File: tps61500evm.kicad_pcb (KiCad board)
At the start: 2 copper layers, 46 x 25 mm, 18 parts, among them J1 Vin, J2 PWM, J3 OVP_Resistor(R1), J4 EN_DIMC, J5 LEDs, J6 FB Resistor, U1 TPS61500PWPR

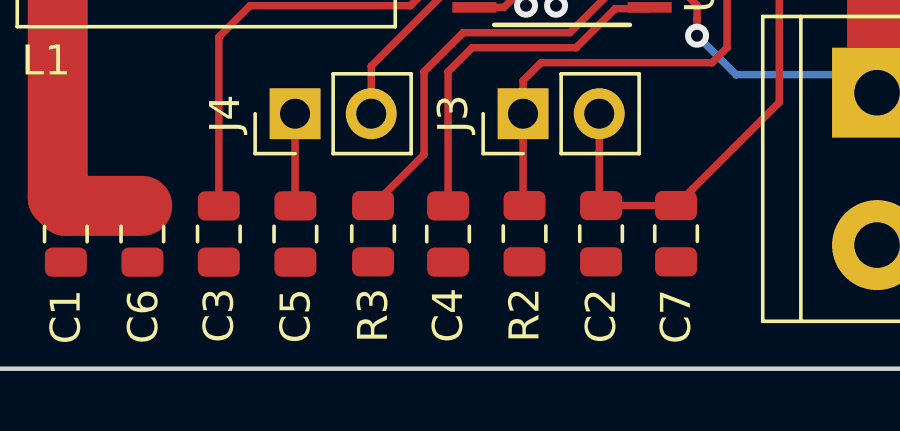
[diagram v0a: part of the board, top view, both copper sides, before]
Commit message: Updated files
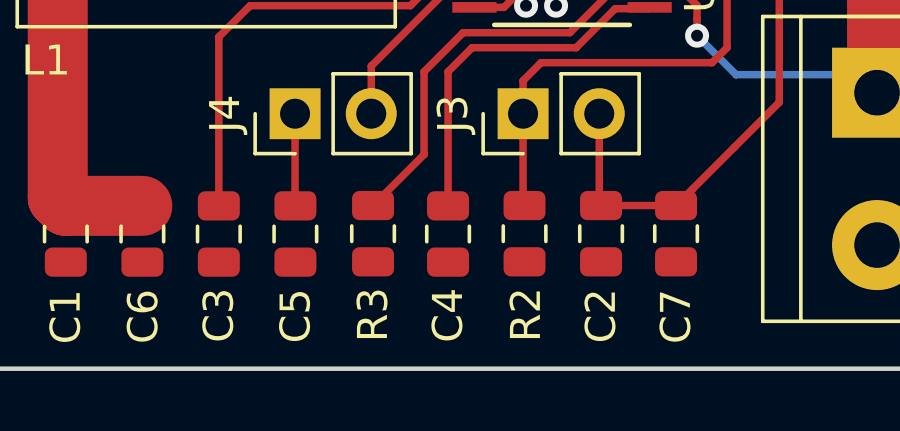
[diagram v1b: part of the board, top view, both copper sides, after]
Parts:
- R2, R3: footprint Capacitor_SMD:C_0805_2012Metric -> Resistor_SMD:R_0805_2012Metric
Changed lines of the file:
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@@
     (add_net "Net-(R3-Pad1)")
+  )
+  (module Resistor_SMD:R_0805_2012Metric (layer F.Cu)
+    (at 45.3 35.5 270)
+    (descr "Resistor SMD 0805 (2012 Metric), square (rectangular) end terminal, IPC_7351 nominal, (Body size source: https://docs.google.com/spreadsheets/d/1BsfQQcO9C6DZCsRaXUlFlo91Tg2WpOkGARC1WS5S8t0/edit?usp=sharing), generated with kicad-footprint-generator")
+    (tags resistor)
+    (attr smd)
+    (fp_text reference R3 (at 2.7 0 270) (layer F.SilkS)
+      (effects (font (size 1 1) (thickness 0.15)))
+    )
+    (fp_text value 33k (at 0 1.65 270) (layer F.Fab)
+      (effects (font (size 1 1) (thickness 0.15)))
+    )
+    (fp_text user %R (at 0 0 270) (layer F.Fab)
+      (effects (font (size 0.5 0.5) (thickness 0.08)))
+    )
+    (fp_line (start 1.68 0.95) (end -1.68 0.95) (layer F.CrtYd) (width 0.05))
+    (fp_line (start 1.68 -0.95) (end 1.68 0.95) (layer F.CrtYd) (width 0.05))
+    (fp_line (start -1.68 -0.95) (end 1.68 -0.95) (layer F.CrtYd) (width 0.05))
+    (fp_line (start -1.68 0.95) (end -1.68 -0.95) (layer F.CrtYd) (width 0.05))
+    (fp_line (start -0.258578 0.71) (end 0.258578 0.71) (layer F.SilkS) (width 0.12))
+    (fp_line (start -0.258578 -0.71) (end 0.258578 -0.71) (layer F.SilkS) (width 0.12))
+    (fp_line (start 1 0.6) (end -1 0.6) (layer F.Fab) (width 0.1))
+    (fp_line (start 1 -0.6) (end 1 0.6) (layer F.Fab) (width 0.1))
+    (fp_line (start -1 -0.6) (end 1 -0.6) (layer F.Fab) (width 0.1))
+    (fp_line (start -1 0.6) (end -1 -0.6) (layer F.Fab) (width 0.1))
+    (pad 2 smd roundrect (at 0.9375 0 270) (size 0.975 1.4) (layers F.Cu F.Paste F.Mask) (roundrect_rratio 0.25)
+      (net 1 GND))
+    (pad 1 smd roundrect (at -0.9375 0 270) (size 0.975 1.4) (layers F.Cu F.Paste F.Mask) (roundrect_rratio 0.25)
+      (net 10 "Net-(R3-Pad1)"))
+    (model ${KISYS3DMOD}/Resistor_SMD.3dshapes/R_0805_2012Metric.wrl
+      (at (xyz 0 0 0))
+      (scale (xyz 1 1 1))
+      (rotate (xyz 0 0 0))
+    )
+  )
+  (module Resistor_SMD:R_0805_2012Metric (layer F.Cu)
+    (at 50.35 35.5 270)
+    (descr "Resistor SMD 0805 (2012 Metric), square (rectangular) end terminal, IPC_7351 nominal, (Body size source: https://docs.google.com/spreadsheets/d/1BsfQQcO9C6DZCsRaXUlFlo91Tg2WpOkGARC1WS5S8t0/edit?usp=sharing), generated with kicad-footprint-generator")
+    (tags resistor)
+    (attr smd)
+    (fp_text reference R2 (at 2.7 -0.05 270) (layer F.SilkS)
+      (effects (font (size 1 1) (thickness 0.15)))
+    )
+    (fp_text value 10k (at 0 1.65 270) (layer F.Fab)
+      (effects (font (size 1 1) (thickness 0.15)))
+    )
+    (fp_line (start -1 0.6) (end -1 -0.6) (layer F.Fab) (width 0.1))
+    (fp_line (start -1 -0.6) (end 1 -0.6) (layer F.Fab) (width 0.1))
+    (fp_line (start 1 -0.6) (end 1 0.6) (layer F.Fab) (width 0.1))
+    (fp_line (start 1 0.6) (end -1 0.6) (layer F.Fab) (width 0.1))
+    (fp_line (start -0.258578 -0.71) (end 0.258578 -0.71) (layer F.SilkS) (width 0.12))
+    (fp_line (start -0.258578 0.71) (end 0.258578 0.71) (layer F.SilkS) (width 0.12))
+    (fp_line (start -1.68 0.95) (end -1.68 -0.95) (layer F.CrtYd) (width 0.05))
+    (fp_line (start -1.68 -0.95) (end 1.68 -0.95) (layer F.CrtYd) (width 0.05))
+    (fp_line (start 1.68 -0.95) (end 1.68 0.95) (layer F.CrtYd) (width 0.05))
+    (fp_line (start 1.68 0.95) (end -1.68 0.95) (layer F.CrtYd) (width 0.05))
+    (fp_text user %R (at 0 0 270) (layer F.Fab)
+      (effects (font (size 0.5 0.5) (thickness 0.08)))
+    )
+    (pad 1 smd roundrect (at -0.9375 0 270) (size 0.975 1.4) (layers F.Cu F.Paste F.Mask) (roundrect_rratio 0.25)
+      (net 11 /OVP))
+    (pad 2 smd roundrect (at 0.9375 0 270) (size 0.975 1.4) (layers F.Cu F.Paste F.Mask) (roundrect_rratio 0.25)
+      (net 1 GND))
+    (model ${KISYS3DMOD}/Resistor_SMD.3dshapes/R_0805_2012Metric.wrl
+      (at (xyz 0 0 0))
+      (scale (xyz 1 1 1))
+      (rotate (xyz 0 0 0))
+    )
   )
   (module TPS61500PWPR:SOP65P640X120-15N (layer F.Cu)
@@
     (pad 2 smd roundrect (at 0.9375 0 270) (size 0.975 1.4) (layers F.Cu F.Paste F.Mask) (roundrect_rratio 0.25)
       (net 1 GND))
-    (model ${KISYS3DMOD}/Capacitor_SMD.3dshapes/C_0805_2012Metric.wrl
-      (at (xyz 0 0 0))
-      (scale (xyz 1 1 1))
-      (rotate (xyz 0 0 0))
-    )
-  )
-  (module Capacitor_SMD:C_0805_2012Metric (layer F.Cu)
-    (at 45.3 35.5 270)
-    (descr "Capacitor SMD 0805 (2012 Metric), square (rectangular) end terminal, IPC_7351 nominal, (Body size source: https://docs.google.com/spreadsheets/d/1BsfQQcO9C6DZCsRaXUlFlo91Tg2WpOkGARC1WS5S8t0/edit?usp=sharing), generated with kicad-footprint-generator")
-    (tags capacitor)
-    (attr smd)
-    (fp_text reference R3 (at 2.72 0 270) (layer F.SilkS)
-      (effects (font (size 1 1) (thickness 0.15)))
-    )
-    (fp_text value 33k (at 0 1.65 270) (layer F.Fab)
-      (effects (font (size 1 1) (thickness 0.15)))
-    )
-    (fp_text user %R (at 0 0 270) (layer F.Fab)
-      (effects (font (size 0.5 0.5) (thickness 0.08)))
-    )
-    (fp_line (start 1.68 0.95) (end -1.68 0.95) (layer F.CrtYd) (width 0.05))
-    (fp_line (start 1.68 -0.95) (end 1.68 0.95) (layer F.CrtYd) (width 0.05))
-    (fp_line (start -1.68 -0.95) (end 1.68 -0.95) (layer F.CrtYd) (width 0.05))
-    (fp_line (start -1.68 0.95) (end -1.68 -0.95) (layer F.CrtYd) (width 0.05))
-    (fp_line (start -0.258578 0.71) (end 0.258578 0.71) (layer F.SilkS) (width 0.12))
-    (fp_line (start -0.258578 -0.71) (end 0.258578 -0.71) (layer F.SilkS) (width 0.12))
-    (fp_line (start 1 0.6) (end -1 0.6) (layer F.Fab) (width 0.1))
-    (fp_line (start 1 -0.6) (end 1 0.6) (layer F.Fab) (width 0.1))
-    (fp_line (start -1 -0.6) (end 1 -0.6) (layer F.Fab) (width 0.1))
-    (fp_line (start -1 0.6) (end -1 -0.6) (layer F.Fab) (width 0.1))
-    (pad 2 smd roundrect (at 0.9375 0 270) (size 0.975 1.4) (layers F.Cu F.Paste F.Mask) (roundrect_rratio 0.25)
-      (net 1 GND))
-    (pad 1 smd roundrect (at -0.9375 0 270) (size 0.975 1.4) (layers F.Cu F.Paste F.Mask) (roundrect_rratio 0.25)
-      (net 10 "Net-(R3-Pad1)"))
-    (model ${KISYS3DMOD}/Capacitor_SMD.3dshapes/C_0805_2012Metric.wrl
-      (at (xyz 0 0 0))
-      (scale (xyz 1 1 1))
-      (rotate (xyz 0 0 0))
-    )
-  )
-  (module Capacitor_SMD:C_0805_2012Metric (layer F.Cu)
-    (at 50.35 35.5 270)
-    (descr "Capacitor SMD 0805 (2012 Metric), square (rectangular) end terminal, IPC_7351 nominal, (Body size source: https://docs.google.com/spreadsheets/d/1BsfQQcO9C6DZCsRaXUlFlo91Tg2WpOkGARC1WS5S8t0/edit?usp=sharing), generated with kicad-footprint-generator")
-    (tags capacitor)
-    (attr smd)
-    (fp_text reference R2 (at 2.71 0 270) (layer F.SilkS)
-      (effects (font (size 1 1) (thickness 0.15)))
-    )
-    (fp_text value 10k (at 0 1.65 270) (layer F.Fab)
-      (effects (font (size 1 1) (thickness 0.15)))
-    )
-    (fp_line (start -1 0.6) (end -1 -0.6) (layer F.Fab) (width 0.1))
-    (fp_line (start -1 -0.6) (end 1 -0.6) (layer F.Fab) (width 0.1))
-    (fp_line (start 1 -0.6) (end 1 0.6) (layer F.Fab) (width 0.1))
-    (fp_line (start 1 0.6) (end -1 0.6) (layer F.Fab) (width 0.1))
-    (fp_line (start -0.258578 -0.71) (end 0.258578 -0.71) (layer F.SilkS) (width 0.12))
-    (fp_line (start -0.258578 0.71) (end 0.258578 0.71) (layer F.SilkS) (width 0.12))
-    (fp_line (start -1.68 0.95) (end -1.68 -0.95) (layer F.CrtYd) (width 0.05))
-    (fp_line (start -1.68 -0.95) (end 1.68 -0.95) (layer F.CrtYd) (width 0.05))
-    (fp_line (start 1.68 -0.95) (end 1.68 0.95) (layer F.CrtYd) (width 0.05))
-    (fp_line (start 1.68 0.95) (end -1.68 0.95) (layer F.CrtYd) (width 0.05))
-    (fp_text user %R (at 0 0 270) (layer F.Fab)
-      (effects (font (size 0.5 0.5) (thickness 0.08)))
-    )
-    (pad 1 smd roundrect (at -0.9375 0 270) (size 0.975 1.4) (layers F.Cu F.Paste F.Mask) (roundrect_rratio 0.25)
-      (net 11 /OVP))
-    (pad 2 smd roundrect (at 0.9375 0 270) (size 0.975 1.4) (layers F.Cu F.Paste F.Mask) (roundrect_rratio 0.25)
-      (net 1 GND))
